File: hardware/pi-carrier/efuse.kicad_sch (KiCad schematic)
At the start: 9 parts, among them U13 TPS2421-1DDAR

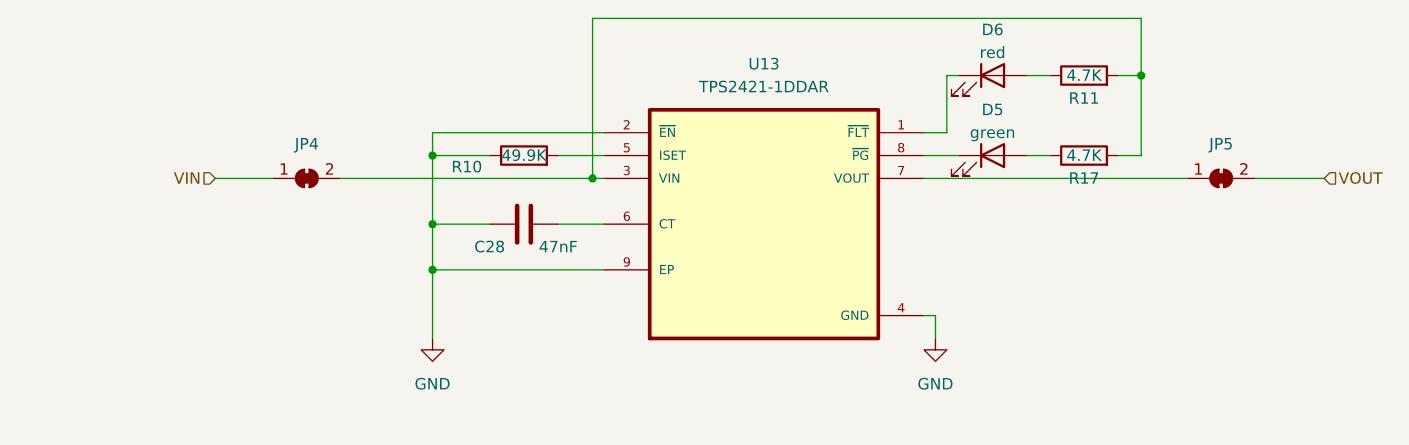
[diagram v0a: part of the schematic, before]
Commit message: pi-carrier: rework efuse layout
Proble: efuse chip is upside-down.

Right the chip and add power layers to improve power routing, in and out.
Drop jumpers as they are no longer needed.
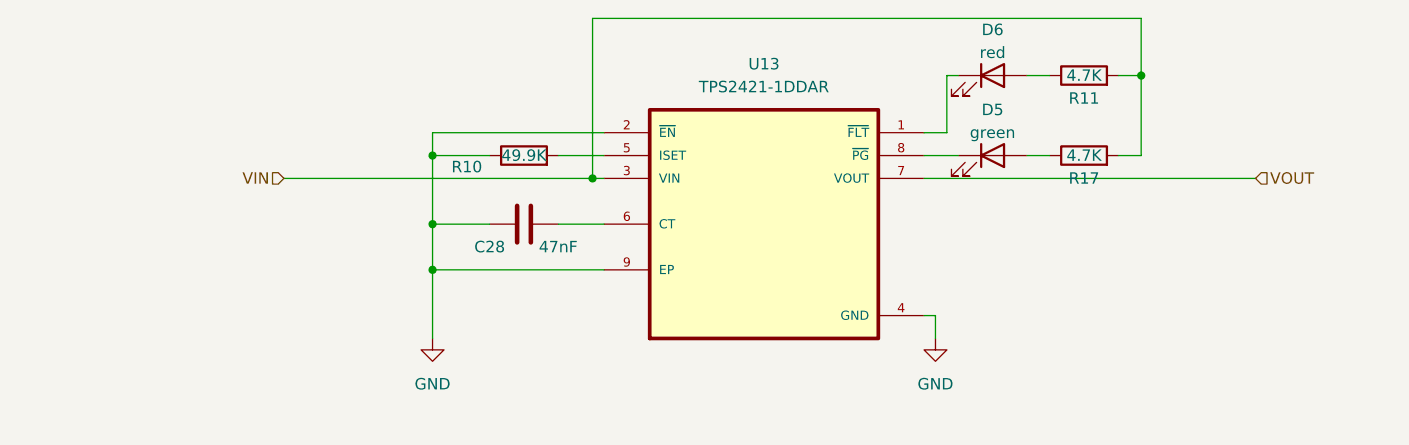
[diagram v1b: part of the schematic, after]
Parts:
- removed JP4, JP5: SolderJumper_2_Bridged, Jumper:SolderJumper-2_P1.3mm_Bridged_RoundedPad1.0x1.5mm, symbol Jumper:SolderJumper_2_Bridged
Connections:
- net VIN: now also R11.2, R17.2, U13.3 (VIN)
- net VOUT: now also U13.7 (VOUT)
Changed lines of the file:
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@@
     (stroke (width 0) (type default))
   )
-  (wire (pts (xy 176.53 85.09) (xy 205.74 85.09))
+  (wire (pts (xy 176.53 85.09) (xy 213.36 85.09))
     (stroke (width 0) (type default))
   )
@@
     (stroke (width 0) (type default))
   )
-  (wire (pts (xy 111.76 85.09) (xy 139.7 85.09))
+  (wire (pts (xy 105.41 85.09) (xy 139.7 85.09))
     (stroke (width 0) (type default))
   )
@@
     (stroke (width 0) (type default))
   )
-  (wire (pts (xy 97.79 85.09) (xy 104.14 85.09))
-    (stroke (width 0) (type default))
-  )
   (wire (pts (xy 198.12 82.55) (xy 200.66 82.55))
     (stroke (width 0) (type default))
   )
   (wire (pts (xy 121.92 82.55) (xy 128.27 82.55))
-    (stroke (width 0) (type default))
-  )
-  (wire (pts (xy 213.36 85.09) (xy 220.98 85.09))
     (stroke (width 0) (type default))
   )
@@
     (effects (font (size 1.27 1.27)) (justify left bottom))
   )
-  (hierarchical_label "VOUT" (shape input) (at 220.98 85.09 0) (fields_autoplaced)
+  (hierarchical_label "VOUT" (shape input) (at 213.36 85.09 0) (fields_autoplaced)
     (effects (font (size 1.27 1.27)) (justify left))
   )
-  (hierarchical_label "VIN" (shape input) (at 97.79 85.09 180) (fields_autoplaced)
+  (hierarchical_label "VIN" (shape input) (at 105.41 85.09 180) (fields_autoplaced)
     (effects (font (size 1.27 1.27)) (justify right))
   )
@@
     )
   )
-  (symbol (lib_id "Jumper:SolderJumper_2_Bridged") (at 107.95 85.09 0) (unit 1)
-    (in_bom yes) (on_board yes) (dnp no) (fields_autoplaced)
-    (property "Reference" "JP4" (at 107.95 81.28 0)
-      (effects (font (size 1.27 1.27)))
-    )
-    (property "Value" "SolderJumper_2_Bridged" (at 107.95 81.28 0)
-      (effects (font (size 1.27 1.27)) hide)
-    )
-    (property "Footprint" "Jumper:SolderJumper-2_P1.3mm_Bridged_RoundedPad1.0x1.5mm" (at 107.95 85.09 0)
-      (effects (font (size 1.27 1.27)) hide)
-    )
-    (property "Datasheet" "~" (at 107.95 85.09 0)
-      (effects (font (size 1.27 1.27)) hide)
-    )
-    (pin "1")
-    (pin "2")
-    (instances
-      (project "eurocard"
-        (path "/e048be62-6e5d-4330-8748-f1a6c1c5d89d/4dfe9b43-7b43-4154-be91-1074449c60f9"
-          (reference "JP4") (unit 1)
-        )
-      )
-    )
-  )
   (symbol (lib_id "00_eurocard:TPS2421-1DDAR") (at 158.75 90.17 0) (unit 1)
     (in_bom yes) (on_board yes) (dnp no) (fields_autoplaced)
@@
         )
       )
-    )
-  )
-  (symbol (lib_id "Jumper:SolderJumper_2_Bridged") (at 209.55 85.09 0) (unit 1)
-    (in_bom yes) (on_board yes) (dnp no) (fields_autoplaced)
-    (property "Reference" "JP5" (at 209.55 81.28 0)
-      (effects (font (size 1.27 1.27)))
-    )
-    (property "Value" "SolderJumper_2_Bridged" (at 209.55 81.28 0)
-      (effects (font (size 1.27 1.27)) hide)
-    )
-    (property "Footprint" "Jumper:SolderJumper-2_P1.3mm_Bridged_RoundedPad1.0x1.5mm" (at 209.55 85.09 0)
-      (effects (font (size 1.27 1.27)) hide)
-    )
-    (property "Datasheet" "~" (at 209.55 85.09 0)
-      (effects (font (size 1.27 1.27)) hide)
-    )
-    (pin "1")
-    (pin "2")
-    (instances
-      (project "eurocard"
-        (path "/e048be62-6e5d-4330-8748-f1a6c1c5d89d/4dfe9b43-7b43-4154-be91-1074449c60f9"
-          (reference "JP5") (unit 1)
-        )
-      )

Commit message: pi-carrier: update to version 4
Problem: design files and board skil still says v3.2.

Bump to v4.

Also change some schematic page sizes from A4 to US letter.
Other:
- company: (none) -> WorlickWerx
- title: (none) -> Molliebus Pi Carrier
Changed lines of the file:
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@@
 (kicad_sch (version 20230121) (generator eeschema)
-  (paper "A4")
+  (paper "USLetter")
+  (title_block
+    (title "Molliebus Pi Carrier")
+    (date "2024-04-20")
+    (rev "4")
+    (company "WorlickWerx")
+    (comment 1 "SPDX-License-Identifier: CERN-OHL-1.2")
+  )
   (junction (at 121.92 90.17) (diameter 0) (color 0 0 0 0)
   )
